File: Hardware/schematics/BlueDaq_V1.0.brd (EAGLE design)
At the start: 67.2 x 72 mm, 75 parts, among them IC1 MEGA8-AI, Q1 MMBT2222, Q2 MMBT2222, Q3 MMBT2222, Q4 MMBT2222, U1 MCP73831, U2 TPS61200, U3 BME280, U4 MIC5225-3.3, U5 MIC5219 5V, X1 USB-MICROB, X2 3.5mm, X4 3.5mm, Y1 16 mhz

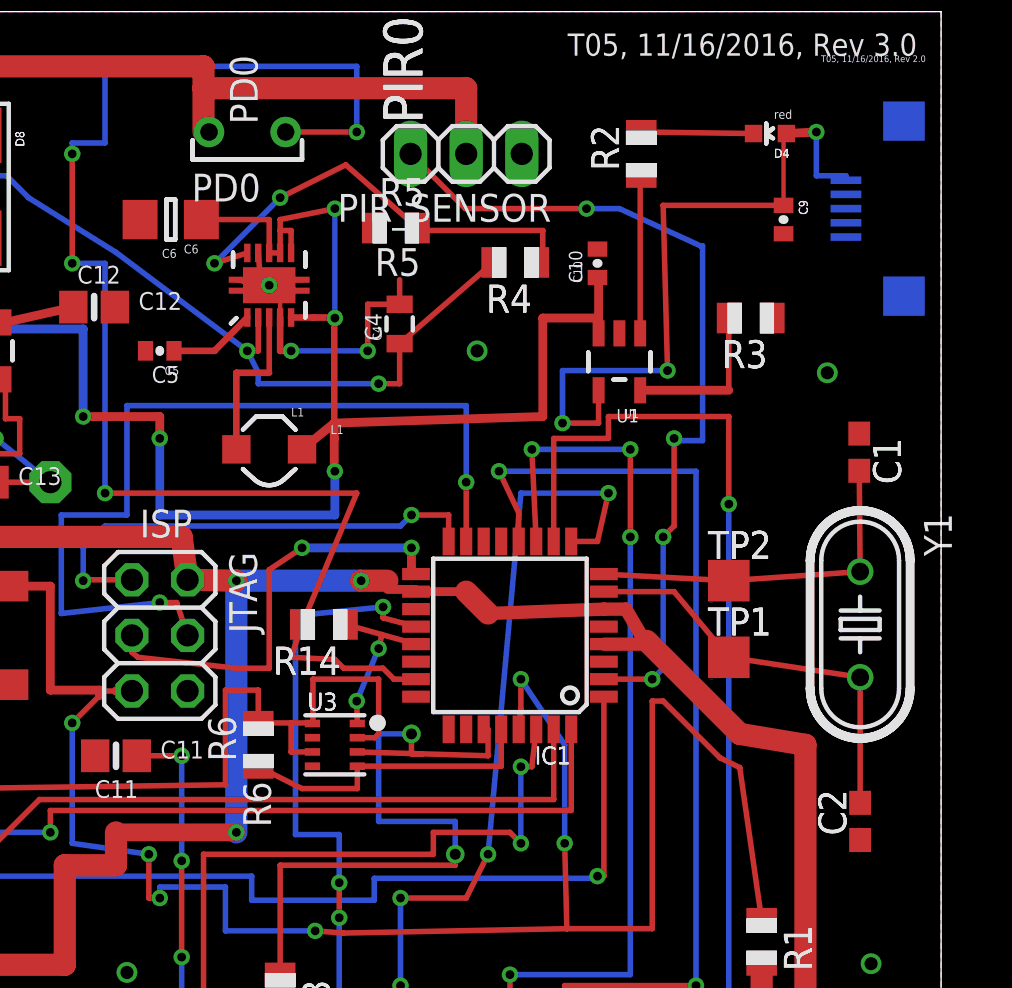
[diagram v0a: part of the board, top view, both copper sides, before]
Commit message: oh no fix
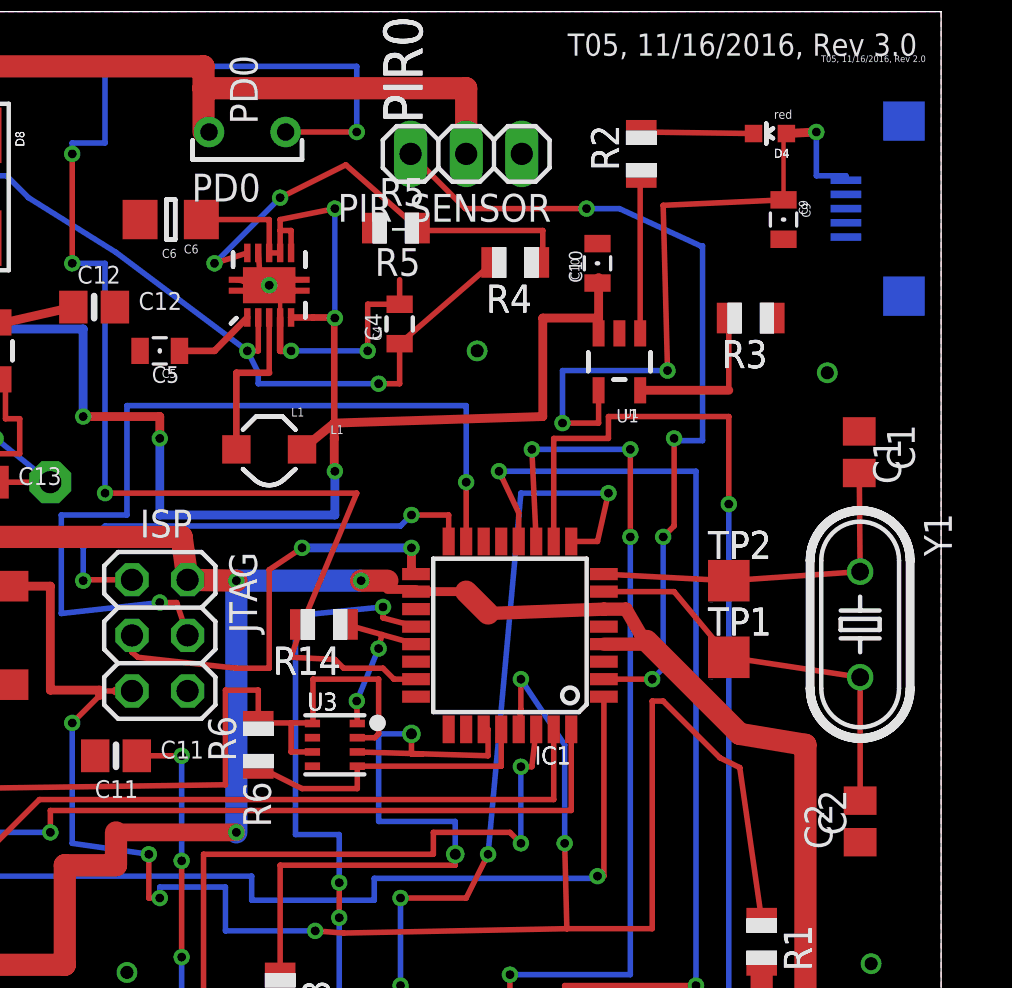
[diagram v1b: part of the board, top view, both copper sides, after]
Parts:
- C1, C2: device rcl:C0603 -> rcl:C0805
- C10, C5, C9: device SparkFun:0402-CAP -> SparkFun:0805
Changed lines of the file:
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@@
 <element name="+9V" library="adafruit" package="1X01" value="" x="19.5" y="50.5" rot="MR0"/>
 <element name="-9V" library="adafruit" package="1X01" value="" x="26.5" y="50.5" rot="MR0"/>
-<element name="C1" library="rcl" package="C0603" value="22p" x="63.46" y="51.87" rot="R270"/>
-<element name="C10" library="SparkFun" package="0402-CAP" value="4.7uF" x="51.5" y="60.5" rot="R90"/>
+<element name="C1" library="rcl" package="C0805" value="22p" x="63.46" y="51.87" rot="R270"/>
+<element name="C10" library="SparkFun" package="0805" value="4.7uF" x="51.5" y="60.5" rot="R90"/>
 <element name="C12" library="microbuilder" package="0805-NO@1" value=".1uF" x="28.5" y="58.5"/>
-<element name="C2" library="rcl" package="C0603" value="22p" x="63.5" y="35" rot="R90"/>
+<element name="C2" library="rcl" package="C0805" value="22p" x="63.5" y="35" rot="R90"/>
 <element name="C4" library="CH_passive" package="0805" value="22uF" x="42.46" y="57.73" rot="R90"/>
-<element name="C5" library="SparkFun" package="0402-CAP" value="0.1uF" x="31.5" y="56.5" rot="R180"/>
+<element name="C5" library="SparkFun" package="0805" value="0.1uF" x="31.5" y="56.5" rot="R180"/>
 <element name="C6" library="CH_passive" package="1206" value="10uF" x="32" y="62.5" rot="R180"/>
 <element name="C7" library="microbuilder" package="0805-NO@1" value="10uF" x="13.5" y="60.5"/>
 <element name="C8" library="microbuilder" package="0805-NO@1" value="10uF" x="15.5" y="54" rot="R270"/>
-<element name="C9" library="SparkFun" package="0402-CAP" value="4.7uF" x="60" y="62.5" rot="R270"/>
+<element name="C9" library="SparkFun" package="0805" value="4.7uF" x="60" y="62.5" rot="R270"/>
 <element name="D1" library="microbuilder" package="SOD-323" value="1N4148" x="30.5" y="19.5" rot="R90"/>
 <element name="D2" library="microbuilder" package="CHIPLED_0805_NOOUTLINE" value="GREEN" x="23.46" y="22.29" rot="R90"/>
@@
 <contactref element="TP1" pad="TP"/>
 <wire x1="57.5" y1="42.5" x2="63.5" y2="41.587" width="0.254" layer="1"/>
-<wire x1="63.5" y1="35.85" x2="63.5" y2="41.587" width="0.254" layer="1"/>
+<wire x1="63.5" y1="35.95" x2="63.5" y2="41.587" width="0.254" layer="1"/>
 <wire x1="57.5" y1="42.5" x2="55" y2="45.5" width="0.254" layer="1"/>
 <wire x1="55" y1="45.5" x2="51.7926" y2="45.5" width="0.254" layer="1"/>
@@
 <contactref element="IC1" pad="8"/>
 <contactref element="TP2" pad="TP"/>
-<wire x1="63.46" y1="51.02" x2="63.5" y2="46.413" width="0.254" layer="1"/>
+<wire x1="63.46" y1="50.92" x2="63.5" y2="46.413" width="0.254" layer="1"/>
 <wire x1="63.5" y1="46.413" x2="57.5" y2="46" width="0.254" layer="1"/>
 <wire x1="57.5" y1="46" x2="51.7926" y2="46.3" width="0.254" layer="1"/>
@@
 <wire x1="51.55" y1="57.3001" x2="51.55" y2="58" width="0.4064" layer="1"/>
 <wire x1="51.55" y1="58" x2="51.55" y2="59.85" width="0.4064" layer="1"/>
-<wire x1="51.55" y1="59.85" x2="51.5" y2="59.85" width="0.254" layer="1"/>
+<wire x1="51.55" y1="59.85" x2="51.5" y2="59.6" width="0.254" layer="1"/>
 <wire x1="7.33" y1="41.75" x2="12.5" y2="41.83" width="0.4064" layer="16"/>
 <wire x1="12.5" y1="41.83" x2="12.5" y2="57.5" width="0.4064" layer="16"/>
@@
 <contactref element="C5" pad="1"/>
 <contactref element="U2" pad="1"/>
-<wire x1="32.15" y1="56.5" x2="34" y2="56.5" width="0.3048" layer="1"/>
+<wire x1="32.4" y1="56.5" x2="34" y2="56.5" width="0.3048" layer="1"/>
 <wire x1="34" y1="56.5" x2="35.5" y2="58.025" width="0.3048" layer="1"/>
 </signal>
@@
 <via x="61.5" y="66.5" extent="1-16" drill="0.4"/>
 <wire x1="60" y1="66.43" x2="60.13" y2="66.43" width="0.4064" layer="1"/>
-<wire x1="60" y1="66.43" x2="60" y2="63.15" width="0.2032" layer="1"/>
+<wire x1="60" y1="66.43" x2="60" y2="63.4" width="0.2032" layer="1"/>
 <wire x1="61.5" y1="66.5" x2="61.5" y2="64.5" width="0.254" layer="16"/>
 <wire x1="61.5" y1="64.5" x2="62.85" y2="64.5" width="0.254" layer="16"/>
 <wire x1="62.85" y1="64.5" x2="62.85" y2="64.3" width="0.254" layer="16"/>
 <contactref element="U1" pad="4"/>
-<wire x1="60" y1="63.15" x2="54.5" y2="63.15" width="0.254" layer="1"/>
+<wire x1="60" y1="63.4" x2="54.5" y2="63.15" width="0.254" layer="1"/>
 <wire x1="54.5" y1="63.15" x2="54.7" y2="55.6" width="0.254" layer="1"/>
 <via x="54.7" y="55.6" extent="1-16" drill="0.4"/>
